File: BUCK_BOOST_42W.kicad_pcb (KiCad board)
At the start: 4 copper layers, 207 x 108 mm, 226 parts, among them J1 Conn_01x08_Pin, J10 Conn_01x04_Pin, J11 Conn_01x04_Pin, J12 Conn_01x04_Pin, J13 Conn_01x12_Socket, J14 Conn_01x16_Socket, J15 Conn_01x02_Pin, J16 Conn_01x02_Pin, J17 Conn_01x02_Pin, J2 Conn_01x03_Pin, J3 Conn_01x04_Pin, J4 Conn_01x04_Pin, J5 Conn_01x04_Pin, J6 Conn_01x04_Pin, J7 Conn_01x04_Pin, J8 Conn_01x04_Pin, J9 Conn_01x04_Pin, Q1 BSC0902NSI, Q2 BSC0902NSI, Q3 BSC0902NSI, Q4 BSC0902NSI, Q5 2N3904, U1 INA226, U10 INA226, U11 INA226, U12 INA226, U13 INA226, U14 INA226, U15 INA226, U16 INA226, U2 INA226, U3 INA226, U4 INA226, U5 LM5176RHF, U6 TPS563201, U7 INA226, U8 INA226, U9 INA226

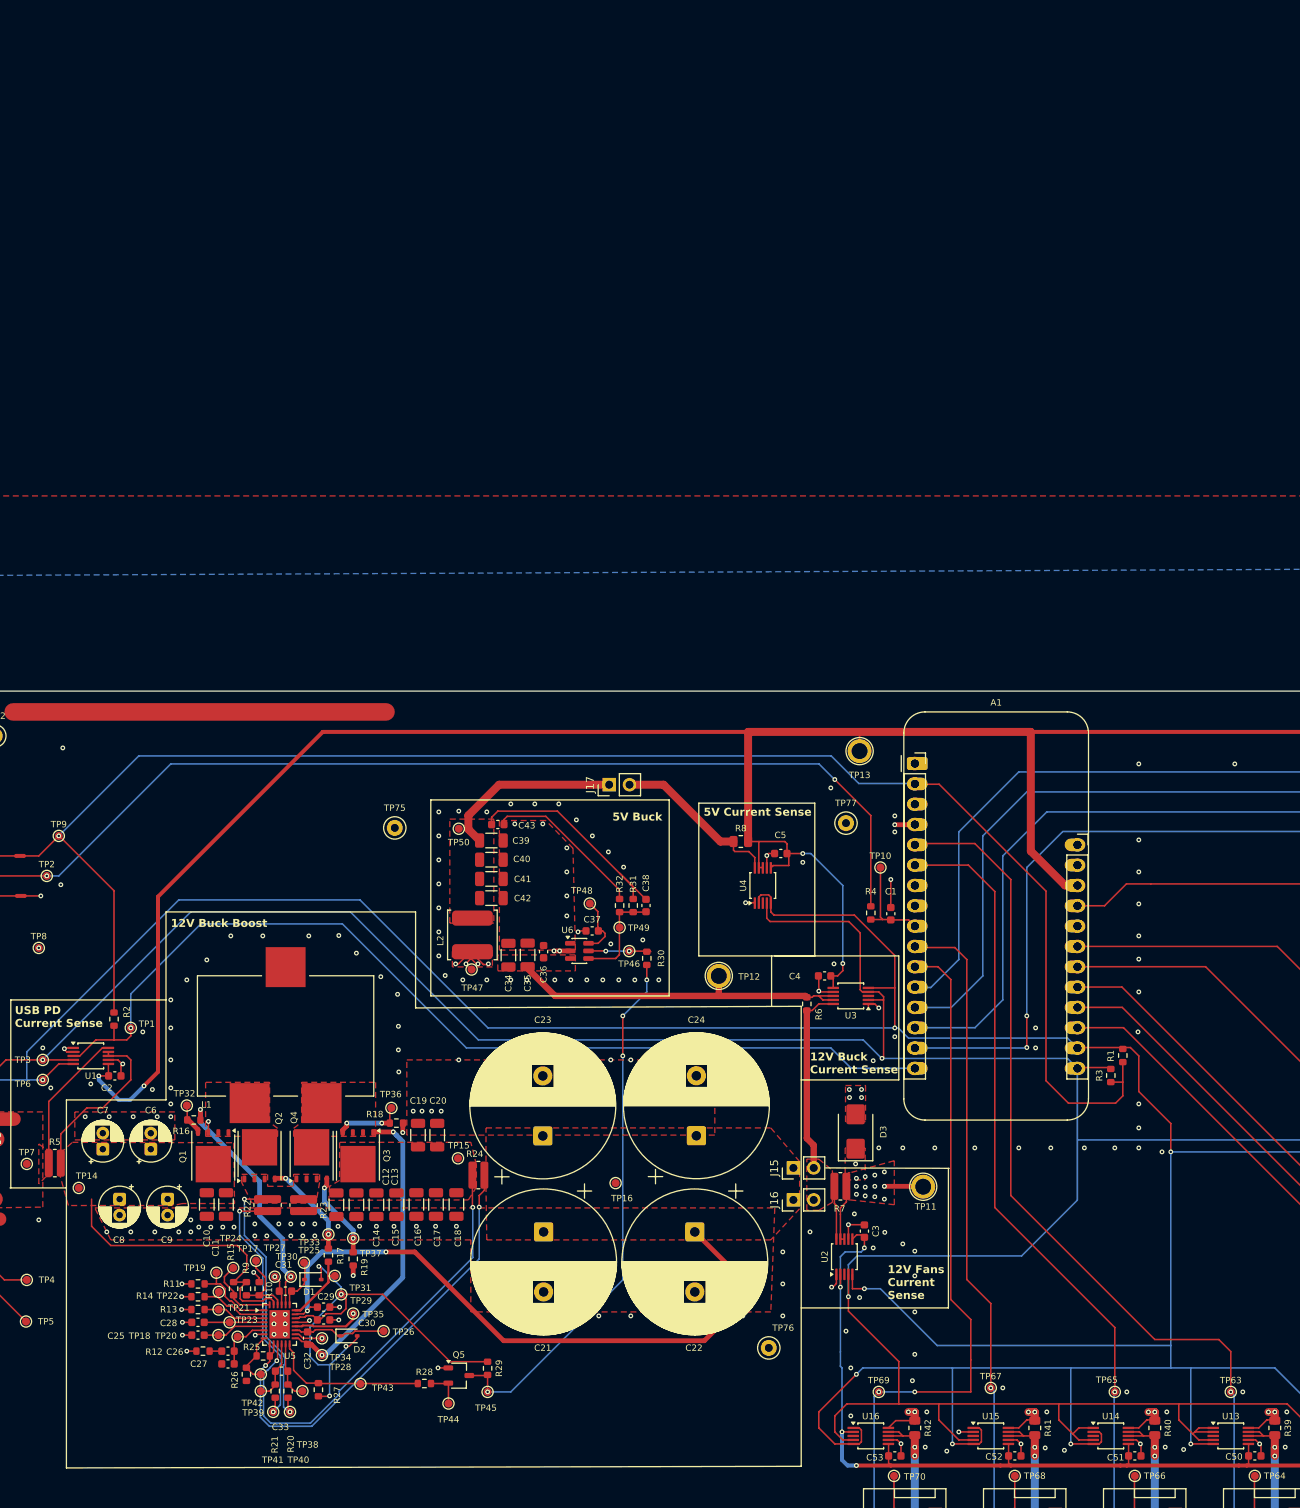
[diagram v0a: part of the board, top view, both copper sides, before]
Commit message: sense resistor partial changes
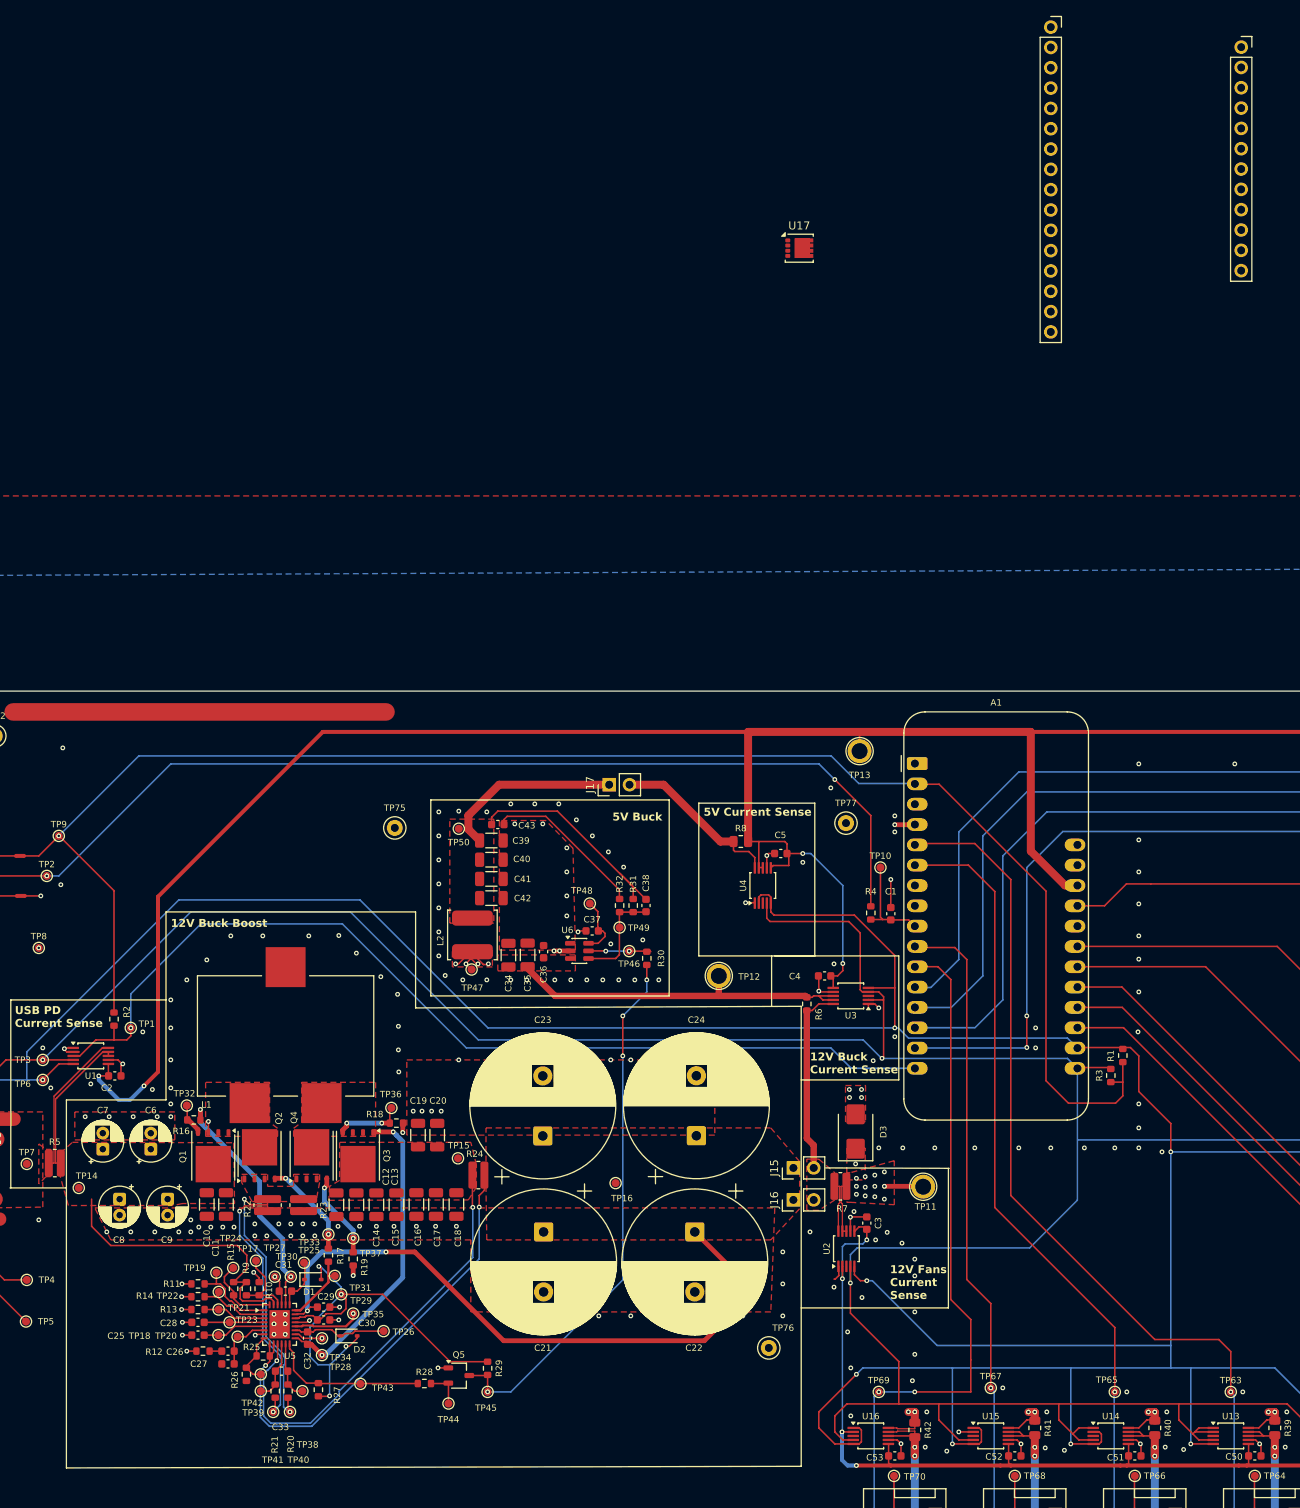
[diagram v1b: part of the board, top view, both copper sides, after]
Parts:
- added U17: CSD25402Q3A, Package_SON:VSON-8_3.3x3.3mm_P0.65mm_NexFET, F.Cu at (138.6, -18.0)
- moved J13 101.8 mm to (193.8, -43.1)
- moved J14 93.6 mm to (170.0, -45.6)
- moved C3 1.04 mm to (147.0, 103.9)
- moved U2 1.03 mm to (144.4, 107.1)
- moved R42 0.25 mm to (153.0, 129.8)
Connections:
- net Net-(Q2-S-Pad1) renamed /Buck_Boost/Vshunt+
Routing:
- net /USB_PD: track 58.5 -> 55.5 mm
- net /fan10/V_fan: track 16.4 -> 18.2 mm
- net /5V: track 557.8 -> 558.8 mm
- net /GND: track 190.3 -> 191.3 mm
- net /Buck_Boost/Vshunt+: track 34.2 -> 35.1 mm
